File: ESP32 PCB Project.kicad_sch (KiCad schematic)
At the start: 9 parts, among them SW1 SW_Push, U1 ESP32-S3-WROOM-1, U2 AMS1117-3.3

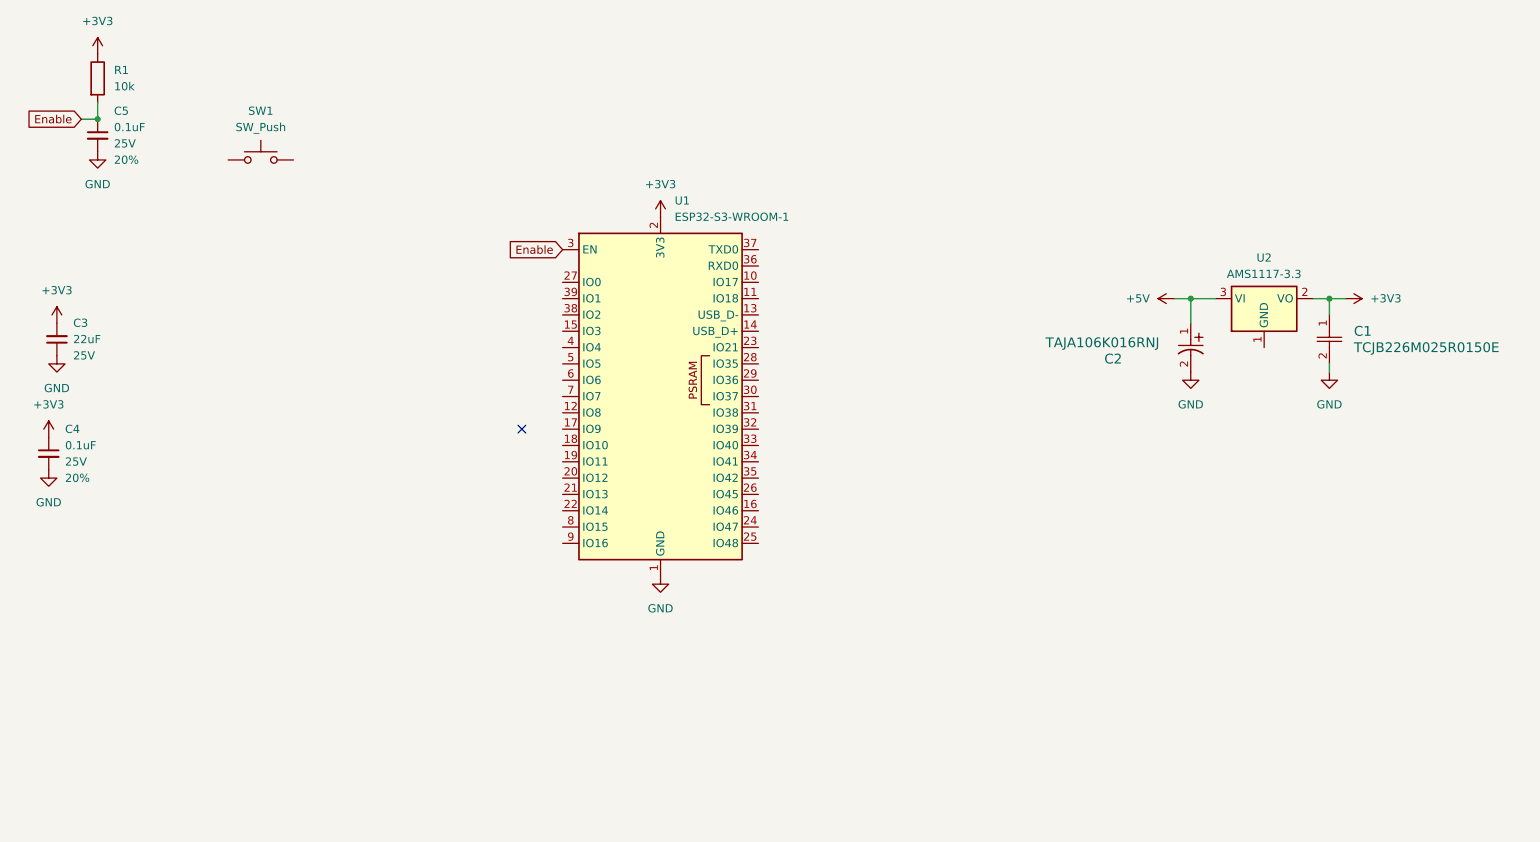
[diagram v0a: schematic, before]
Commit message: update
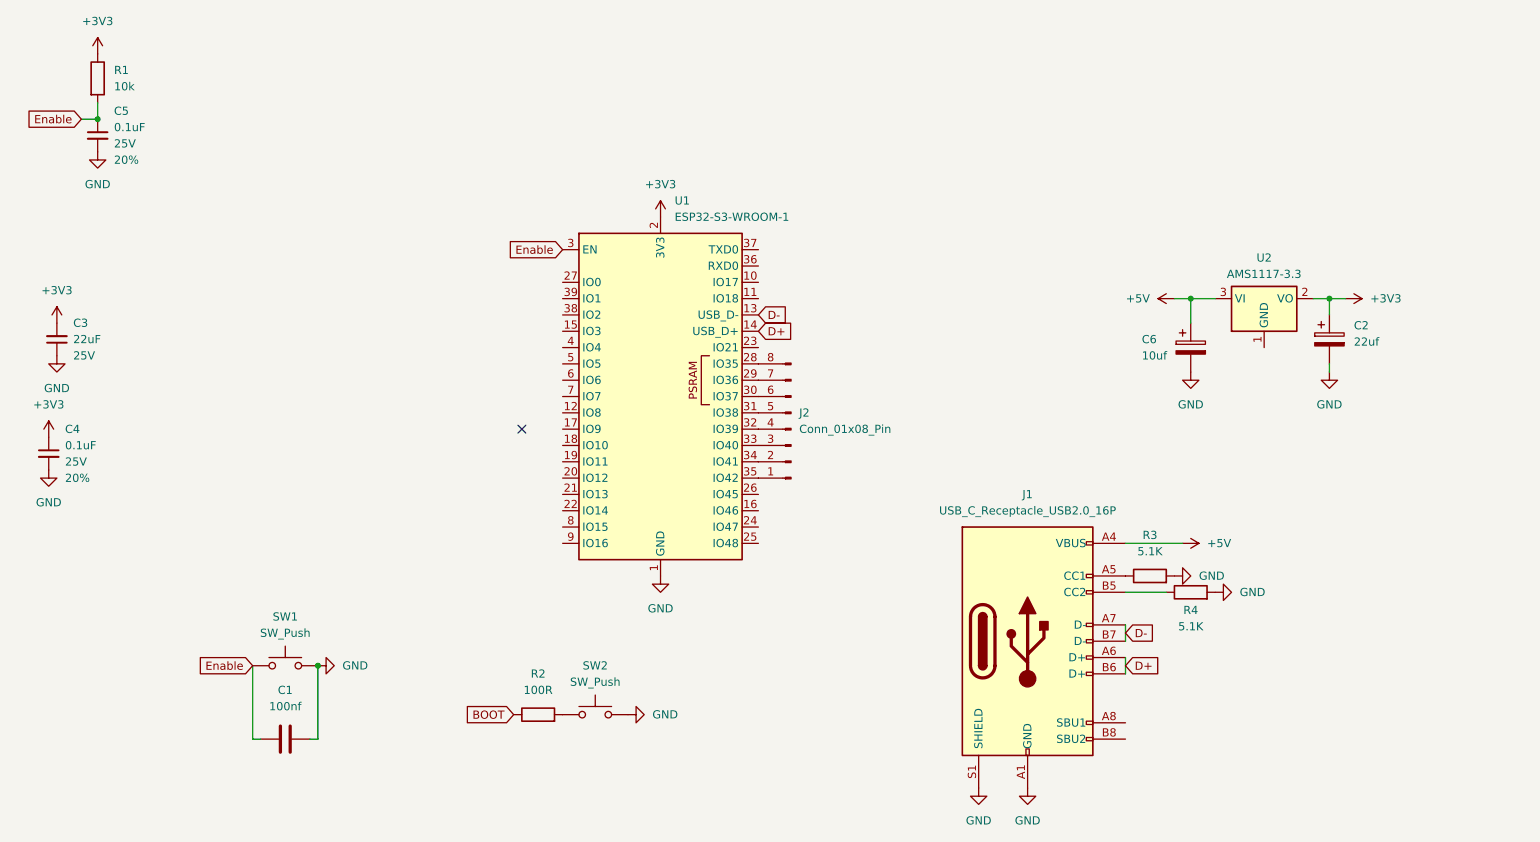
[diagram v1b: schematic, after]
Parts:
- removed C1: TCJB226M025R0150E, CAP_TCJ_B_KAV, symbol TCJB226M025R0150E:TCJB226M025R0150E
- removed C2: TAJA106K016RNJ, TAJA_AVX, symbol TAJA106K016RNJ:TAJA106K016RNJ
- added C1: 100nf, Capacitor_SMD:C_0201_0603Metric, symbol Device:C
- added C2: 22uf, Capacitor_Tantalum_SMD:CP_EIA-1608-08_AVX-J, symbol Device:C_Polarized
- added C6: 10uf, Capacitor_Tantalum_SMD:CP_EIA-1608-08_AVX-J, symbol Device:C_Polarized
- added J1: USB_C_Receptacle_USB2.0_16P, Connector_USB:USB_C_Receptacle_Amphenol_12401610E4-2A_CircularHoles, symbol Connector:USB_C_Receptacle_USB2.0_16P
- added J2: Conn_01x08_Pin, Connector_PinHeader_1.00mm:PinHeader_1x08_P1.00mm_Vertical, symbol Connector:Conn_01x08_Pin
- added R2: 100R, Resistor_SMD:R_0805_2012Metric, symbol Device:R
- added R3, R4: 5.1K, Resistor_SMD:R_0805_2012Metric, symbol Device:R
- added SW2: SW_Push, Button_Switch_THT:SW_PUSH_6mm, symbol Switch:SW_Push
- C3: footprint PCM_SparkFun-Capacitor:C_0805_2012Metric -> Capacitor_SMD:C_0201_0603Metric
- C4, C5: footprint PCM_SparkFun-Capacitor:C_0603_1608Metric -> Capacitor_SMD:C_0201_0603Metric
- SW1: footprint (none) -> Button_Switch_THT:SW_PUSH_6mm
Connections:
- net +3V3: now also C2.1
- net +5V: now also C6.1, J1.A4 (VBUS), J1.A9 (VBUS), J1.B4 (VBUS), J1.B9 (VBUS)
- net Enable: now also SW1.1, C1.1
- net GND: now also SW1.2, C1.2, C2.2, C6.2, J1.A1 (GND), J1.A12 (GND), J1.B1 (GND), J1.B12 (GND), J1.S1 (SHIELD), R3.2, R4.2, SW2.2
- net D-: now reaches U1.13 (USB_D-)
- net D-: now also J1.A7 (D-), J1.B7 (D-)
- net D+: now reaches U1.14 (USB_D+)
- net D+: now also J1.A6 (D+), J1.B6 (D+)
- net at U1.28 (IO35): now also J2.8 (Pin_8)
- net at U1.29 (IO36): now also J2.7 (Pin_7)
- net at U1.30 (IO37): now also J2.6 (Pin_6)
- net at U1.31 (IO38): now also J2.5 (Pin_5)
- net at U1.32 (IO39): now also J2.4 (Pin_4)
- net at U1.33 (IO40): now also J2.3 (Pin_3)
- net at U1.34 (IO41): now also J2.2 (Pin_2)
- net at U1.35 (IO42): now also J2.1 (Pin_1)
- new net: J1.A5 (CC1), R3.1
- new net: R2.2, SW2.1
- new net: J1.B5 (CC2), R4.1
- new net BOOT: R2.1
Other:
- moved on the sheet: SW1
